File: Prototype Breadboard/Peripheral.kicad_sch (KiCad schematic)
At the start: 26 parts, among them J1 Button, J2 Button, J3 Conn_02x06_Odd_Even_MountingP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, J4 Conn_01x23_MountingPin, J5 Conn_01x23_MountingPin, U9 RP2040, Y1 3225-4P 12MHz

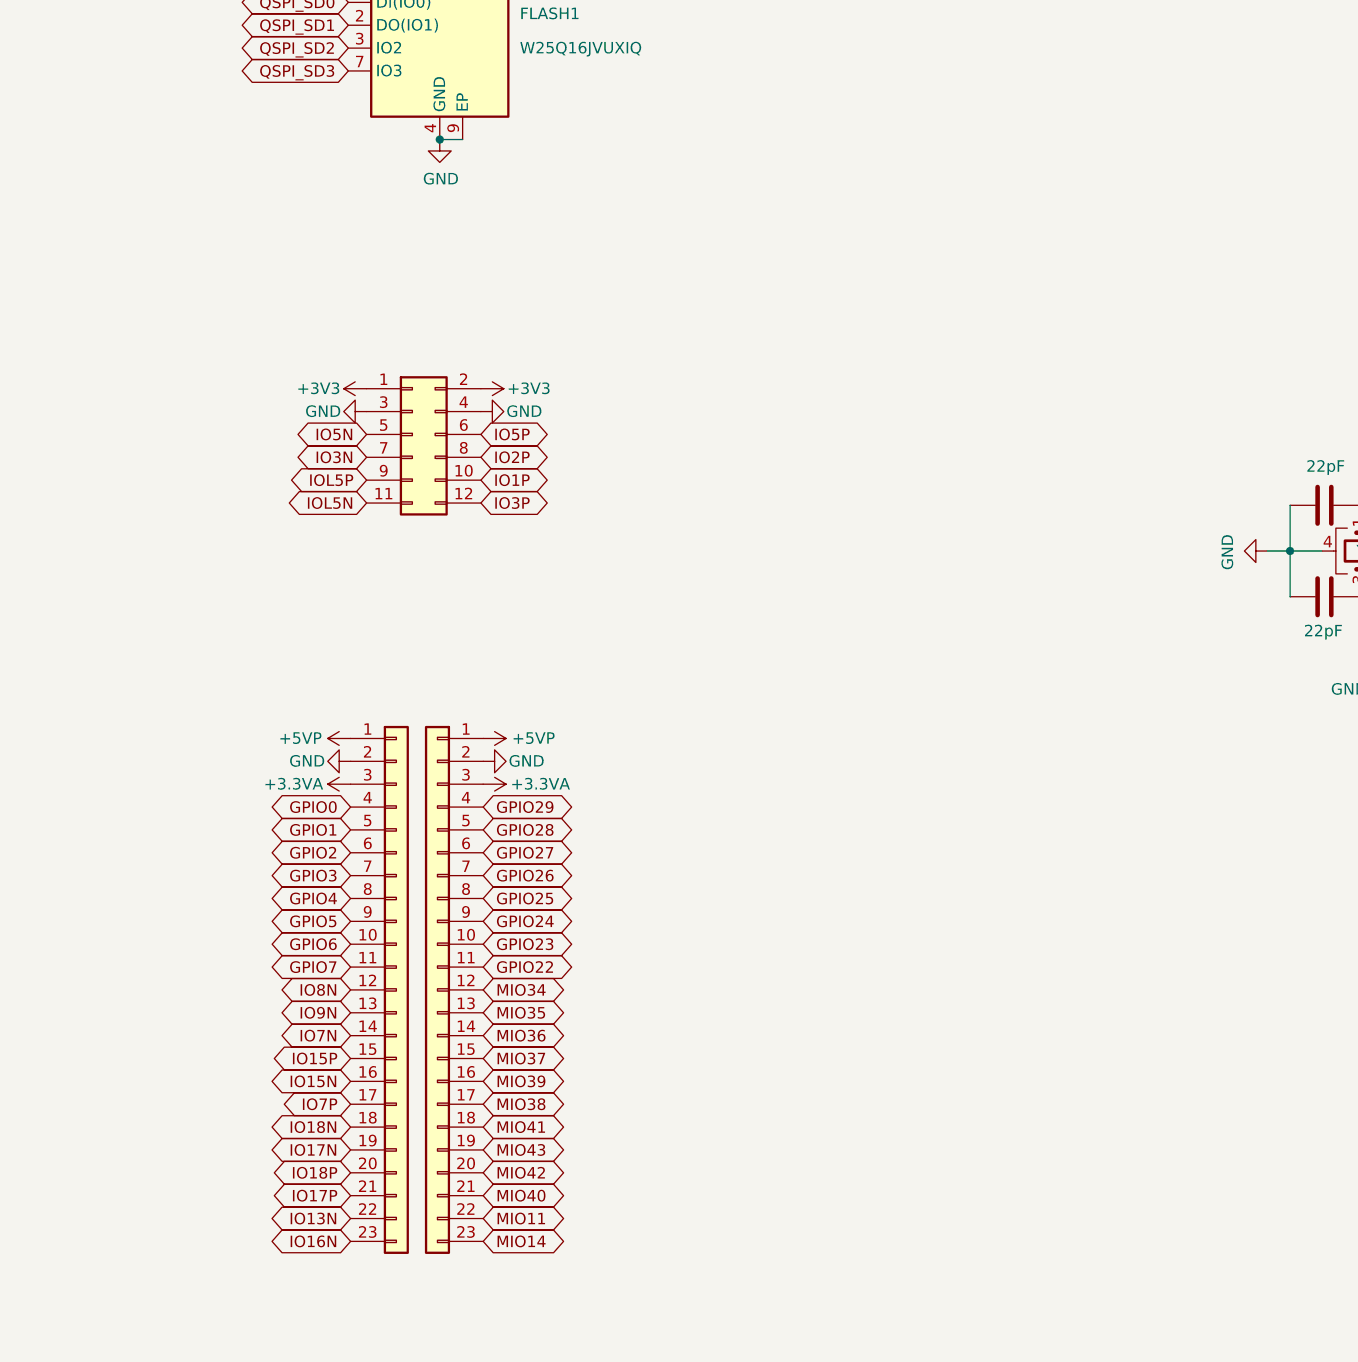
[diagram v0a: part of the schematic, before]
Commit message: 1/4 update
update the breadboard version
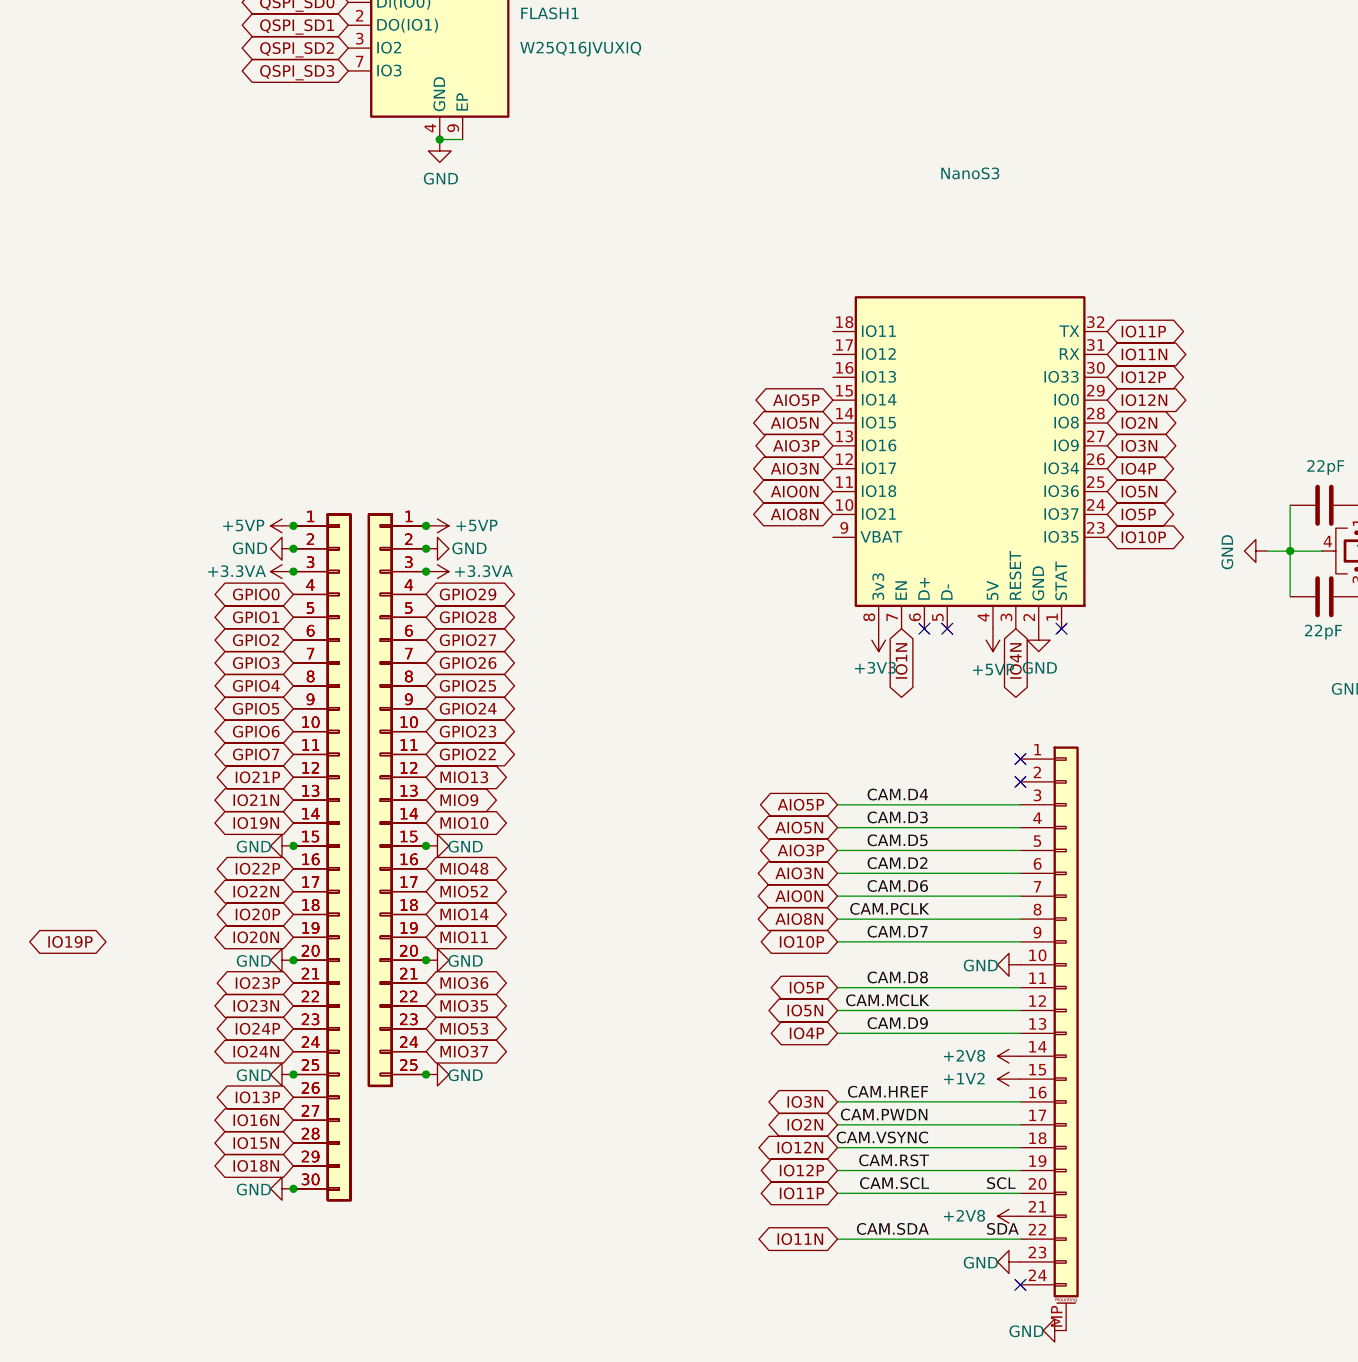
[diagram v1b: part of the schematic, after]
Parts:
- removed J3: Conn_02x06_Odd_Even_MountingPin, Connector_PinSocket_2.54mm:PinSocket_2x06_P2.54mm_Vertical, symbol Connector_Generic_MountingPin:Conn_02x06_Odd_Even_MountingPin
- removed J4, J5: Conn_01x23_MountingPin, Connector_PinHeader_2.54mm:PinHeader_1x23_P2.54mm_Vertical, symbol Connector_Generic_MountingPin:Conn_01x23_MountingPin
- added J3, J7: Conn_01x30_MountingPin, Connector_PinHeader_2.54mm:PinHeader_1x30_P2.54mm_Vertical, symbol Connector_Generic_MountingPin:Conn_01x30_MountingPin
- added J4, J5: Conn_01x25_MountingPin, Connector_PinHeader_2.54mm:PinHeader_1x25_P2.54mm_Vertical, symbol Connector_Generic_MountingPin:Conn_01x25_MountingPin
- added J8: Conn_01x24_MountingPin, Connector_FFC-FPC:TE_2-1734839-4_1x24-1MP_P0.5mm_Horizontal, symbol Connector_Generic_MountingPin:Conn_01x24_MountingPin
- added U10: NanoS3, Sync_VT extras:NanoS3, symbol new shii:NanoS3
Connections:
- net +3.3VA: now also J3.3 (Pin_3), J4.3 (Pin_3), J5.3 (Pin_3), J7.3 (Pin_3)
- net +3V3: now also U10.8 (3v3)
- net +5VP: now also J3.1 (Pin_1), J4.1 (Pin_1), J5.1 (Pin_1), J7.1 (Pin_1), U10.4 (5V)
- net GND: now also J3.15 (Pin_15), J3.2 (Pin_2), J3.20 (Pin_20), J3.25 (Pin_25), J3.30 (Pin_30), J4.15 (Pin_15), J4.2 (Pin_2), J4.20 (Pin_20), J4.25 (Pin_25), J5.15 (Pin_15), J5.2 (Pin_2), J5.20 (Pin_20), J5.25 (Pin_25), J7.15 (Pin_15), J7.2 (Pin_2), J7.20 (Pin_20), J7.25 (Pin_25), J7.30 (Pin_30), J8.10 (Pin_10), J8.23 (Pin_23), J8.MP (MountPin), U10.2 (GND)
- net GPIO0: now also J3.4 (Pin_4), J7.4 (Pin_4)
- net GPIO1: now also J3.5 (Pin_5), J7.5 (Pin_5)
- net GPIO2: now also J3.6 (Pin_6), J7.6 (Pin_6)
- net GPIO22: now also J4.11 (Pin_11), J5.11 (Pin_11)
- net GPIO23: now also J4.10 (Pin_10), J5.10 (Pin_10)
- net GPIO24: now also J4.9 (Pin_9), J5.9 (Pin_9)
- net GPIO25: now also J4.8 (Pin_8), J5.8 (Pin_8)
- net GPIO26: now also J4.7 (Pin_7), J5.7 (Pin_7)
- net GPIO27: now also J4.6 (Pin_6), J5.6 (Pin_6)
- net GPIO28: now also J4.5 (Pin_5), J5.5 (Pin_5)
- net GPIO29: now also J4.4 (Pin_4), J5.4 (Pin_4)
- net GPIO3: now also J3.7 (Pin_7), J7.7 (Pin_7)
- net GPIO4: now also J3.8 (Pin_8), J7.8 (Pin_8)
- net GPIO5: now also J3.9 (Pin_9), J7.9 (Pin_9)
- net GPIO6: now also J3.10 (Pin_10), J7.10 (Pin_10)
- net GPIO7: now also J3.11 (Pin_11), J7.11 (Pin_11)
- net IO15N: now also J3.28 (Pin_28), J7.28 (Pin_28)
- net IO16N: now also J3.27 (Pin_27), J7.27 (Pin_27)
- net IO18N: now also J3.29 (Pin_29), J7.29 (Pin_29)
- net IO3N: now also J8.16 (Pin_16), U10.27 (IO9)
- net IO5N: now also J8.12 (Pin_12), U10.25 (IO36)
- net IO5P: now also J8.11 (Pin_11), U10.24 (IO37)
- net MIO11: now also J4.19 (Pin_19), J5.19 (Pin_19)
- net MIO14: now also J4.18 (Pin_18), J5.18 (Pin_18)
- net MIO35: now also J4.22 (Pin_22), J5.22 (Pin_22)
- net MIO36: now also J4.21 (Pin_21), J5.21 (Pin_21)
- net MIO37: now also J4.24 (Pin_24), J5.24 (Pin_24)
- new net +1V2: J8.15 (Pin_15)
- new net +2V8: J8.14 (Pin_14), J8.21 (Pin_21)
- new net AIO0N: J8.7 (Pin_7), U10.11 (IO18)
- new net AIO3N: J8.6 (Pin_6), U10.12 (IO17)
- new net AIO3P: J8.5 (Pin_5), U10.13 (IO16)
- new net AIO5N: J8.4 (Pin_4), U10.14 (IO15)
- new net AIO5P: J8.3 (Pin_3), U10.15 (IO14)
- new net AIO8N: J8.8 (Pin_8), U10.10 (IO21)
- new net IO10P: J8.9 (Pin_9), U10.23 (IO35)
- new net IO11N: J8.22 (Pin_22), U10.31 (RX)
- new net IO11P: J8.20 (Pin_20), U10.32 (TX)
- new net IO12N: J8.18 (Pin_18), U10.29 (IO0)
- new net IO12P: J8.19 (Pin_19), U10.30 (IO33)
- new net IO13P: J3.26 (Pin_26), J7.26 (Pin_26)
- new net IO19N: J3.14 (Pin_14), J7.14 (Pin_14)
- new net IO1N: U10.7 (EN)
- new net IO20N: J3.19 (Pin_19), J7.19 (Pin_19)
- new net IO20P: J3.18 (Pin_18), J7.18 (Pin_18)
- new net IO21N: J3.13 (Pin_13), J7.13 (Pin_13)
- new net IO21P: J3.12 (Pin_12), J7.12 (Pin_12)
- new net IO22N: J3.17 (Pin_17), J7.17 (Pin_17)
- new net IO22P: J3.16 (Pin_16), J7.16 (Pin_16)
- new net IO23N: J3.22 (Pin_22), J7.22 (Pin_22)
- new net IO23P: J3.21 (Pin_21), J7.21 (Pin_21)
- new net IO24N: J3.24 (Pin_24), J7.24 (Pin_24)
- new net IO24P: J3.23 (Pin_23), J7.23 (Pin_23)
- new net IO2N: J8.17 (Pin_17), U10.28 (IO8)
- new net IO4N: U10.3 (RESET)
- new net IO4P: J8.13 (Pin_13), U10.26 (IO34)
- new net MIO10: J4.14 (Pin_14), J5.14 (Pin_14)
- new net MIO13: J4.12 (Pin_12), J5.12 (Pin_12)
- new net MIO48: J4.16 (Pin_16), J5.16 (Pin_16)
- new net MIO52: J4.17 (Pin_17), J5.17 (Pin_17)
- new net MIO53: J4.23 (Pin_23), J5.23 (Pin_23)
- new net MIO9: J4.13 (Pin_13), J5.13 (Pin_13)
- no-connect marks 0 -> 6
